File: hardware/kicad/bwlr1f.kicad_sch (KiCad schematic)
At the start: 67 parts, among them J1 Conn_01x02, Q2 PMV32UP, Q3 DMG1012UW, U1 BME688, U1 RAK3172-SIP, U2 NBM7100ABQX, U3 ZD24C08A, U5 TPL5110

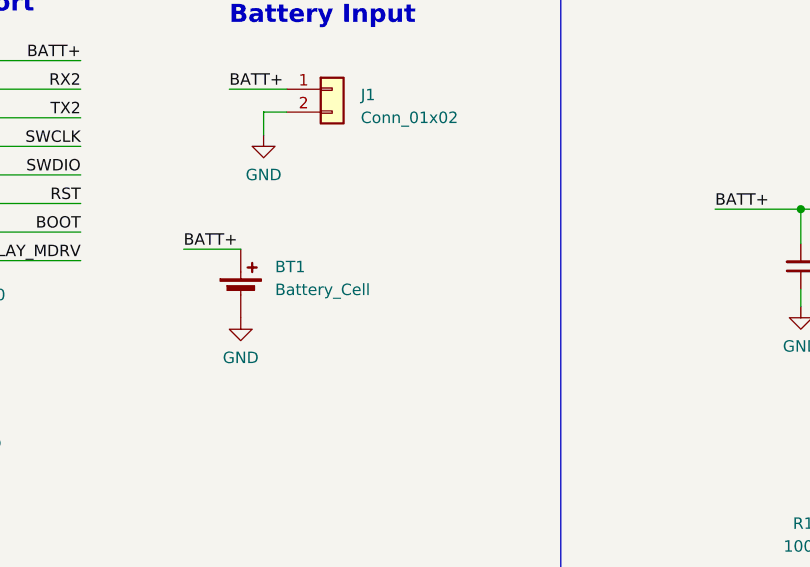
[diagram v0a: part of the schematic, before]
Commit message: Revert "update layout"
This reverts commit 7d4c2235c3ae4d9f911583b993bcb32887b0ae1e.
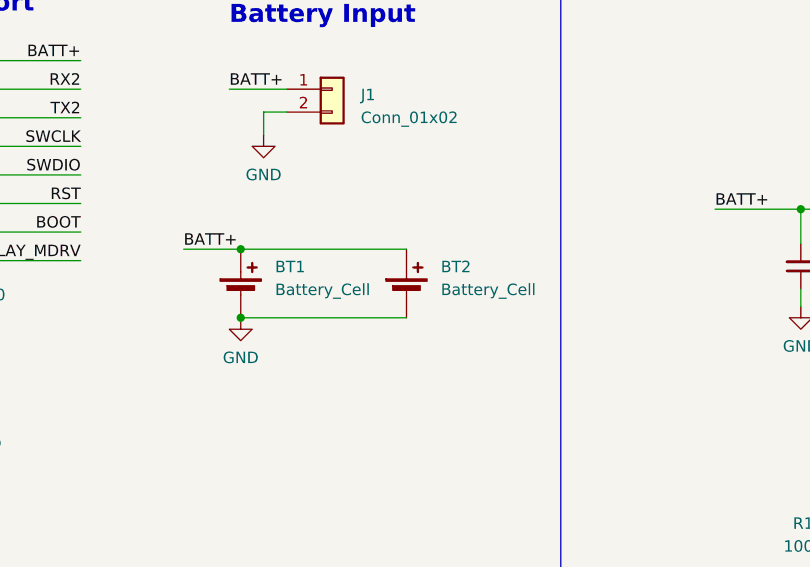
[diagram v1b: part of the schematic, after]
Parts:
- added BT2: Battery_Cell, bwlr1f:BAT-SMD_MY-2032-12, symbol Device:Battery_Cell
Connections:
- net BATT+: now also BT2.1 (+)
- net GND: now also BT2.2 (-)
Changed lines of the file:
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@@
   (junction (at 137.16 226.695) (diameter 0) (color 0 0 0 0)
   )
+  (junction (at 74.93 231.14) (diameter 0) (color 0 0 0 0)
+  )
   (junction (at 50.8 123.825) (diameter 0) (color 0 0 0 0)
   )
@@
   (junction (at 165.1 264.795) (diameter 0) (color 0 0 0 0)
   )
+  (junction (at 74.93 238.76) (diameter 0) (color 0 0 0 0)
+  )
   (junction (at 101.6 64.135) (diameter 0) (color 0 0 0 0)
   )
@@
     (stroke (width 0) (type default))
   )
+  (wire (pts (xy 74.93 231.14) (xy 93.345 231.14))
+    (stroke (width 0) (type default))
+  )
   (wire (pts (xy 157.48 263.525) (xy 157.48 264.795))
     (stroke (width 0) (type default))
@@
     (stroke (width 0) (type default))
   )
+  (wire (pts (xy 74.93 238.76) (xy 93.345 238.76))
+    (stroke (width 0) (type default))
+  )
   (wire (pts (xy 187.325 210.185) (xy 187.325 205.74))
     (stroke (width 0) (type default))
@@
         )
       )
+    )
+  )
+  (symbol (lib_id "Device:Battery_Cell") (at 93.345 236.22 0) (unit 1)
+    (in_bom yes) (on_board yes) (dnp no) (fields_autoplaced)
+    (property "Reference" "BT2" (at 97.155 233.1085 0)
+      (effects (font (size 1.27 1.27)) (justify left))
+    )
+    (property "Value" "Battery_Cell" (at 97.155 235.6485 0)
+      (effects (font (size 1.27 1.27)) (justify left))
+    )
+    (property "Footprint" "bwlr1f:BAT-SMD_MY-2032-12" (at 93.345 234.696 90)
+      (effects (font (size 1.27 1.27)) hide)
+    )
+    (property "Datasheet" "https://datasheet.lcsc.com/lcsc/2012181809_MYOUNG-MY-2032-12_C964833.pdf" (at 93.345 234.696 90)
+      (effects (font (size 1.27 1.27)) hide)
+    )
+    (property "Part Description" "Battery button -25℃~+85℃ CR2032" (at 93.345 236.22 0)
+      (effects (font (size 1.27 1.27)) hide)
+    )
+    (property "Manufacturer" "MYOUNG" (at 93.345 236.22 0)
+      (effects (font (size 1.27 1.27)) hide)
+    )
+    (property "Manufacturer Part Number" "MY-2032-12" (at 93.345 236.22 0)
+      (effects (font (size 1.27 1.27)) hide)
+    )
+    (property "Distributor" "LCSC" (at 93.345 236.22 0)
+      (effects (font (size 1.27 1.27)) hide)
+    )
+    (property "Distributor Part Number" "C964833" (at 93.345 236.22 0)
+      (effects (font (size 1.27 1.27)) hide)
+    )
+    (property "Distributor Link" "https://www.lcsc.com/product-detail/Battery-Connectors_MYOUNG-MY-2032-12_C964833.html" (at 93.345 236.22 0)
+      (effects (font (size 1.27 1.27)) hide)
+    )
+    (pin "1")
+    (pin "2")
+    (instances
+      (project "bwlr1f"
+        (path "/7fec048a-2dfd-4bff-8685-e805b00dfe07"
+          (reference "BT2") (unit 1)
+        )
+      )

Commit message: update layout
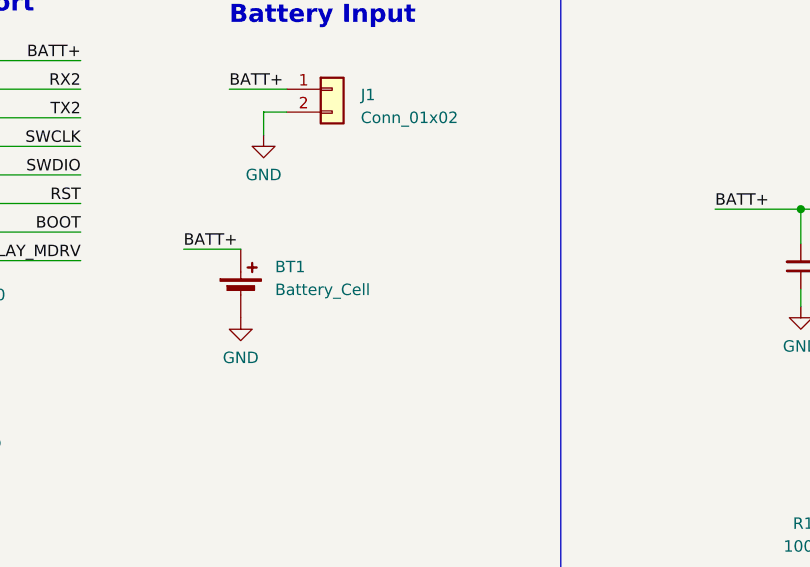
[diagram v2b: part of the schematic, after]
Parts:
- removed BT2: Battery_Cell, bwlr1f:BAT-SMD_MY-2032-12, symbol Device:Battery_Cell
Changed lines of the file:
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@@
   (junction (at 137.16 226.695) (diameter 0) (color 0 0 0 0)
   )
-  (junction (at 74.93 231.14) (diameter 0) (color 0 0 0 0)
-  )
   (junction (at 50.8 123.825) (diameter 0) (color 0 0 0 0)
   )
@@
   (junction (at 165.1 264.795) (diameter 0) (color 0 0 0 0)
   )
-  (junction (at 74.93 238.76) (diameter 0) (color 0 0 0 0)
-  )
   (junction (at 101.6 64.135) (diameter 0) (color 0 0 0 0)
   )
@@
     (stroke (width 0) (type default))
   )
-  (wire (pts (xy 74.93 231.14) (xy 93.345 231.14))
-    (stroke (width 0) (type default))
-  )
   (wire (pts (xy 157.48 263.525) (xy 157.48 264.795))
     (stroke (width 0) (type default))
@@
     (stroke (width 0) (type default))
   )
-  (wire (pts (xy 74.93 238.76) (xy 93.345 238.76))
-    (stroke (width 0) (type default))
-  )
   (wire (pts (xy 187.325 210.185) (xy 187.325 205.74))
     (stroke (width 0) (type default))
@@
         )
       )
-    )
-  )
-  (symbol (lib_id "Device:Battery_Cell") (at 93.345 236.22 0) (unit 1)
-    (in_bom yes) (on_board yes) (dnp no) (fields_autoplaced)
-    (property "Reference" "BT2" (at 97.155 233.1085 0)
-      (effects (font (size 1.27 1.27)) (justify left))
-    )
-    (property "Value" "Battery_Cell" (at 97.155 235.6485 0)
-      (effects (font (size 1.27 1.27)) (justify left))
-    )
-    (property "Footprint" "bwlr1f:BAT-SMD_MY-2032-12" (at 93.345 234.696 90)
-      (effects (font (size 1.27 1.27)) hide)
-    )
-    (property "Datasheet" "https://datasheet.lcsc.com/lcsc/2012181809_MYOUNG-MY-2032-12_C964833.pdf" (at 93.345 234.696 90)
-      (effects (font (size 1.27 1.27)) hide)
-    )
-    (property "Part Description" "Battery button -25℃~+85℃ CR2032" (at 93.345 236.22 0)
-      (effects (font (size 1.27 1.27)) hide)
-    )
-    (property "Manufacturer" "MYOUNG" (at 93.345 236.22 0)
-      (effects (font (size 1.27 1.27)) hide)
-    )
-    (property "Manufacturer Part Number" "MY-2032-12" (at 93.345 236.22 0)
-      (effects (font (size 1.27 1.27)) hide)
-    )
-    (property "Distributor" "LCSC" (at 93.345 236.22 0)
-      (effects (font (size 1.27 1.27)) hide)
-    )
-    (property "Distributor Part Number" "C964833" (at 93.345 236.22 0)
-      (effects (font (size 1.27 1.27)) hide)
-    )
-    (property "Distributor Link" "https://www.lcsc.com/product-detail/Battery-Connectors_MYOUNG-MY-2032-12_C964833.html" (at 93.345 236.22 0)
-      (effects (font (size 1.27 1.27)) hide)
-    )
-    (pin "1")
-    (pin "2")
-    (instances
-      (project "bwlr1f"
-        (path "/7fec048a-2dfd-4bff-8685-e805b00dfe07"
-          (reference "BT2") (unit 1)
-        )
-      )
